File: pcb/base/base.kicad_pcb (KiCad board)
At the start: 2 copper layers, 24 x 24 mm, 21 parts, among them J1 Conn_01x03_Male, J2 Conn_01x03_Male, J3 Conn_01x02_Male, J4 Conn_01x03_Male, U1 STM32F301K6Tx, U2 AP2210-33, U3 tile

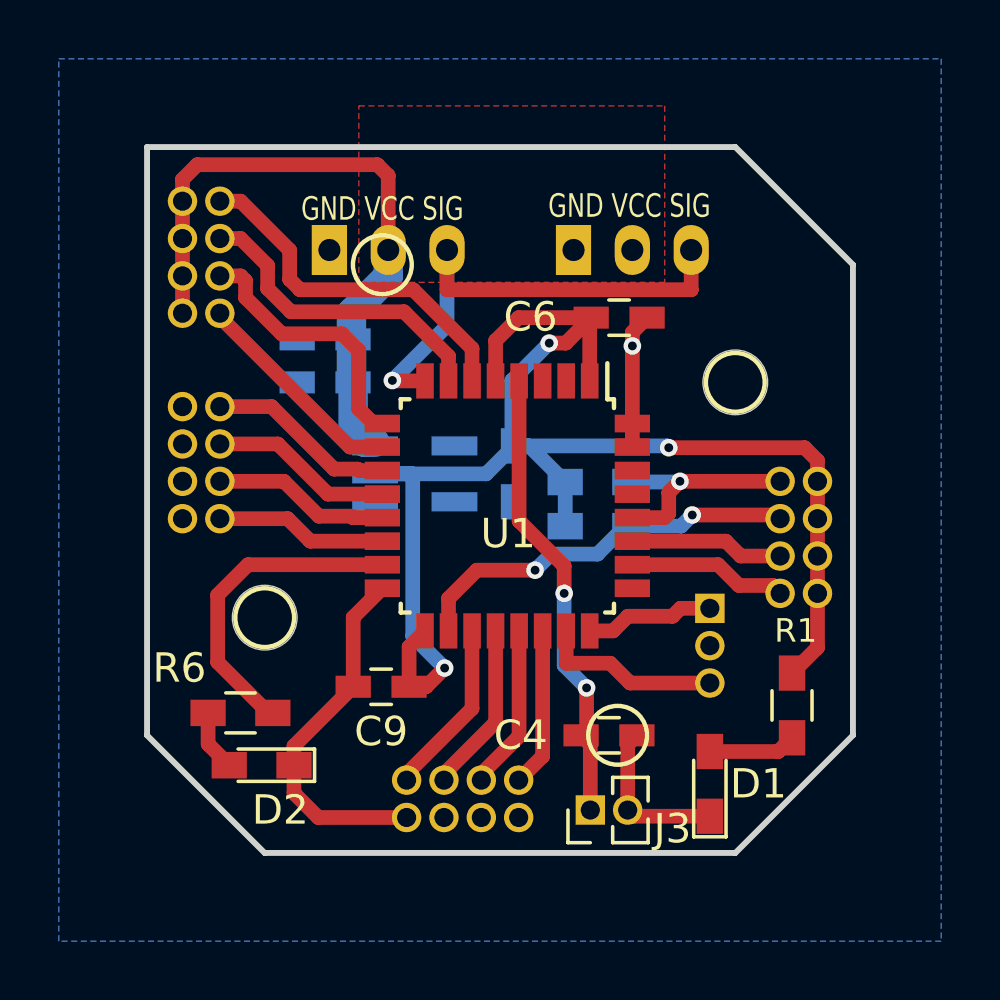
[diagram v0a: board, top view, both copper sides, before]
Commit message: cleaning/upgrades got collection of little modes over sime time, added dxf"
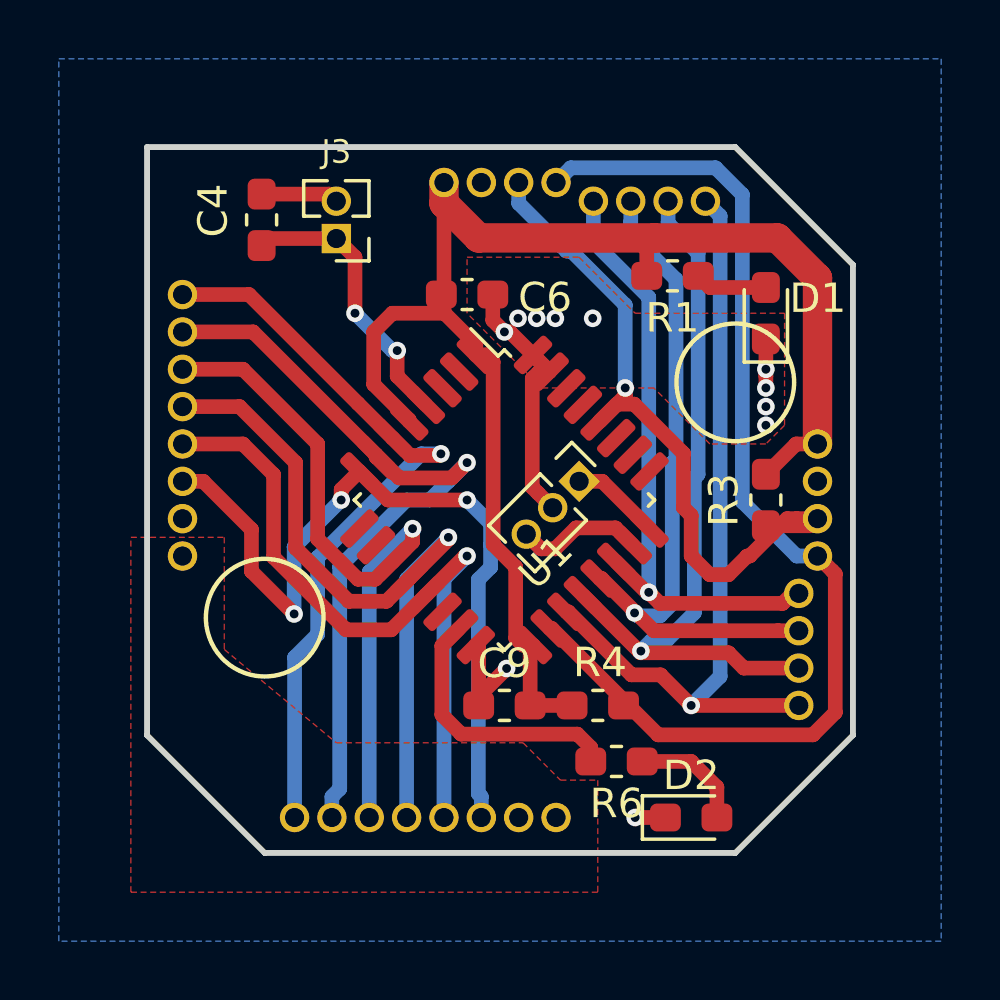
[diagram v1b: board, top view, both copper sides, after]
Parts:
- removed C1: 10uf, Capacitors_SMD:C_0603_HandSoldering
- removed C2, C3: 4.7uf, Capacitors_SMD:C_0603_HandSoldering
- removed Hole1, Hole2: Conn_01x01_Male, Mounting_Holes:MountingHole_2.2mm_M2
- removed J1, J2: Conn_01x03_Male, Connectors_JST:JST_PH_B3B-PH-K_03x2.00mm_Straight
- removed U2: AP2210-33, TO_SOT_Packages_SMD:SOT-23-5_HandSoldering
- C4, C6, C9: footprint Capacitors_SMD:C_0603_HandSoldering -> Capacitor_SMD:C_0603_1608Metric_Pad1.05x0.95mm_HandSolder
- D1, D2: footprint LEDs:LED_0603_HandSoldering -> LED_SMD:LED_0603_1608Metric_Pad1.05x0.95mm_HandSolder
- J3: footprint Pin_Headers:Pin_Header_Straight_1x02_Pitch1.27mm -> Connector_PinHeader_1.27mm:PinHeader_1x02_P1.27mm_Vertical
- J4: footprint Pin_Headers:Pin_Header_Straight_1x03_Pitch1.27mm -> Connector_PinHeader_1.27mm:PinHeader_1x03_P1.27mm_Vertical; moved to F.Cu
- R1, R6: footprint Resistors_SMD:R_0603_HandSoldering -> Resistor_SMD:R_0603_1608Metric_Pad1.05x0.95mm_HandSolder
- R3, R4: footprint Resistors_SMD:R_0603_HandSoldering -> Resistor_SMD:R_0603_1608Metric_Pad1.05x0.95mm_HandSolder; moved to F.Cu
- U1: value STM32F301K6Tx -> STM32G431KBT6; footprint Housings_QFP:LQFP-32_7x7mm_Pitch0.8mm -> Package_QFP:LQFP-32_7x7mm_P0.8mm
- moved J3 21.3 mm to (94.4, 91.1), turned to 180 degrees
- moved C4 21.1 mm to (91.9, 90.5), turned to 270 degrees
- moved D1 16.1 mm to (109.0, 93.7)
- moved R1 15.2 mm to (105.9, 92.4), turned to 180 degrees
- moved D2 14.7 mm to (106.5, 110.8), turned to 0 degrees
- moved R6 12.9 mm to (104.0, 108.9), turned to 180 degrees
- moved J4 6.20 mm to (102.7, 99.4), turned to 315 degrees
- moved R4 6.10 mm to (103.3, 107.0)
- moved R3 5.76 mm to (109.0, 100.0), turned to 90 degrees
- moved C6 5.23 mm to (98.9, 93.0)
- moved C9 4.24 mm to (100.2, 107.0)
- moved U1 0.22 mm to (100.2, 100.0), turned to 315 degrees
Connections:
- U1 pad 10: PA4 -> (no net)
- U1 pad 14: PB0 -> (no net)
- U1 pad 26: PB3 -> (no net)
- U1 pad 27: PB4 -> (no net)
- U1 pad 9: PA3 -> (no net)
- U3 pad 10: I2C_CLK -> GND
- U3 pad 11: PB4 -> BUS
- U3 pad 12: PB3 -> SPI_MOSI
- U3 pad 13: CTX -> SPI_MISO
- U3 pad 14: CRX -> SPI_CLK
- U3 pad 15: USART1_RX -> ADC1
- U3 pad 16: USART1_TX -> ADC0
- U3 pad 2: +3V3 -> GND
- U3 pad 3: +3V3 -> I2C_SDA
- U3 pad 4: +3V3 -> I2C_CLK
- U3 pad 5: GND -> CTX
- U3 pad 6: GND -> CRX
- U3 pad 7: GND -> USART1_RX
- U3 pad 8: GND -> USART1_TX
- U3 pad 9: I2C_SDA -> VCC
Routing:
- net I2C_CLK: track 13.6 -> 37.8 mm, vias 2 -> 0
- net VCC: track 21.9 -> 0.00 mm
- net USART1_TX: track 6.00 -> 27.0 mm, vias 0 -> 1
- net USART1_RX: track 5.80 -> 25.2 mm, vias 0 -> 1
- net SPI_MISO: track 6.23 -> 24.5 mm, vias 0 -> 1
- net SPI_MOSI: track 6.04 -> 24.2 mm, vias 0 -> 1
- net I2C_SDA: track 7.67 -> 25.5 mm
- net CRX: track 5.61 -> 23.4 mm, vias 0 -> 1
- net SPI_CLK: track 6.43 -> 24.1 mm, vias 0 -> 1
- net ADC1: track 10.7 -> 27.2 mm, vias 0 -> 1
- net CTX: track 5.41 -> 21.0 mm, vias 0 -> 1
- net ADC0: track 12.3 -> 25.9 mm, vias 0 -> 1
- net BUS: track 17.3 -> 27.7 mm, vias 1 -> 3
- net PA3: track 9.10 -> 0.00 mm
- net PA4: track 7.48 -> 0.00 mm
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- added copper zone on F.Cu, net GND
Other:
- board text removed: "GND"
- board text removed: "GND VCC SIG"
- board text removed: "SWDIO"
